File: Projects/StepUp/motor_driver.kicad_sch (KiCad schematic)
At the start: 39 parts, among them J4 AST0250404, Q1 BSS84, Q2 2N7002-7-F, U4 TMC2300-LA-T

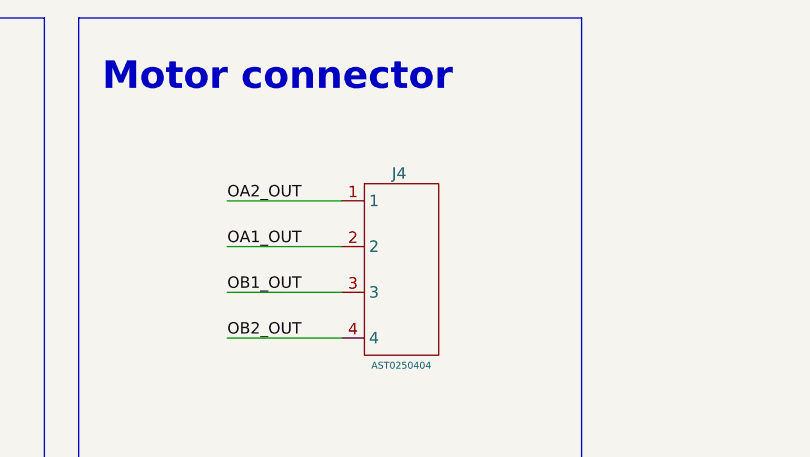
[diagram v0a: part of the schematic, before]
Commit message: feat(v0.3): Layout 90% complete
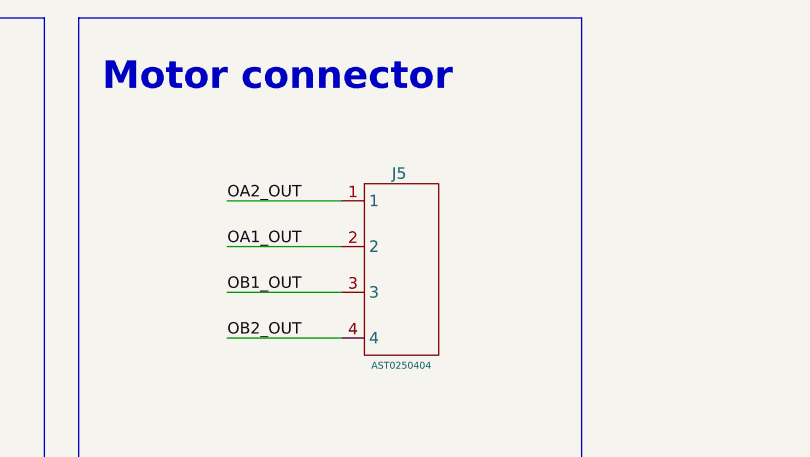
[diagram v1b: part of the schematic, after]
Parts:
- renumbered J4 to J5
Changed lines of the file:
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@@
 		(on_board yes)
 		(dnp no)
-		(property "Reference" "J4"
+		(property "Reference" "J5"
 			(at 142.748 40.132 0)
 			(effects
@@
 			(project "StepUp"
 				(path "/e0cca1c7-c263-49eb-8c40-74000ebe5285/f5cf6bff-0c76-4311-a1f3-856e1fd3b2e7"
-					(reference "J4")
+					(reference "J5")
 					(unit 1)
 				)

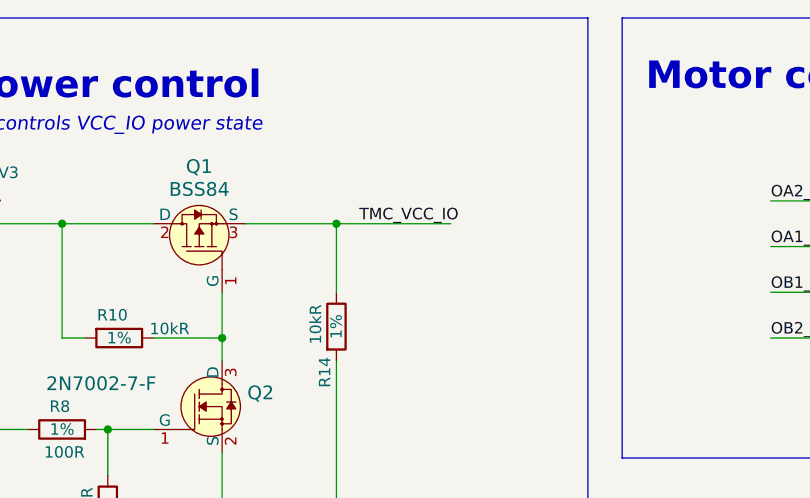
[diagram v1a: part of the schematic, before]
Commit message: feat(v0.3): Files sent to PCBWay for build
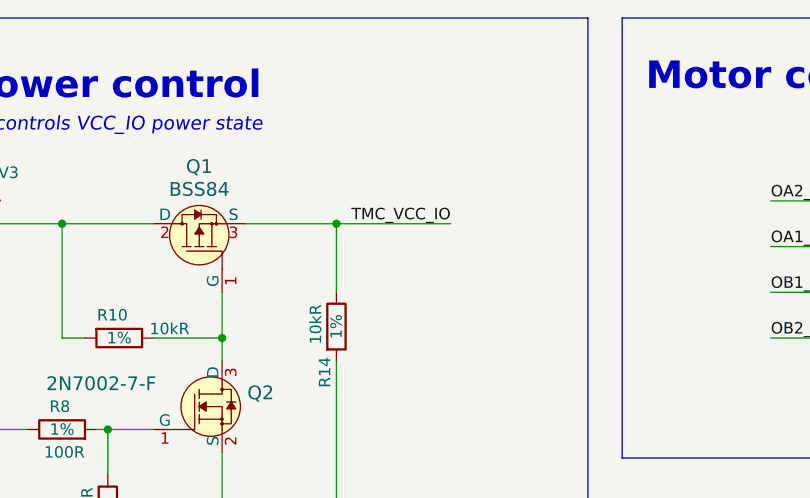
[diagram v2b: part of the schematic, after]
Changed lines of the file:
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@@
-		)
-	)
-	(label "TMC_VCC_IO"
-		(at 78.74 45.72 0)
-		(effects
-			(font
-				(size 1.27 1.27)
-			)
-			(justify left bottom)
 		)
 	)
@@
 		)
 	)
+	(label "TMC_VCC_IO"
+		(at 88.9 45.72 180)
+		(effects
+			(font
+				(size 1.27 1.27)
+			)
+			(justify right bottom)
+		)
+	)
